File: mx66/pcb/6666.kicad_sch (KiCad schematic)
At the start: 145 parts, among them J1 Left side, J2 Right side, K1 100, K10 125, K11 100, K12 100, K13 100, K14 100, K15 125, K16 100, K17 100, K18 100, K19 100, K2 150, K20 125, K21 100, K22 100, K23 100, K24 100, K25 225, K26 100, K27 100, K28 100, K29 100, K3 175, K30 100, K31 100, K32 100, K33 100, K34 100, K35 100, K36 100, K37 100, K38 100, K39 100, K4 225, K40 100, K41 100, K42 100, K43 275, K44 100, K45 100, K46 100, K47 100, K48 125, K49 100, K5 125, K50 100, K51 100, K52 100, K53 125, K54 100, K55 100, K56 100, K57 100, K58 100, K59 100, K6 100, K60 100, K61 100, K62 200, K63 150, K64 225, K65 100, K66 100, K7 100, K8 100, K9 100, U1 MCU_ProMicro_13p, U2 MCU_ProMicro_13p

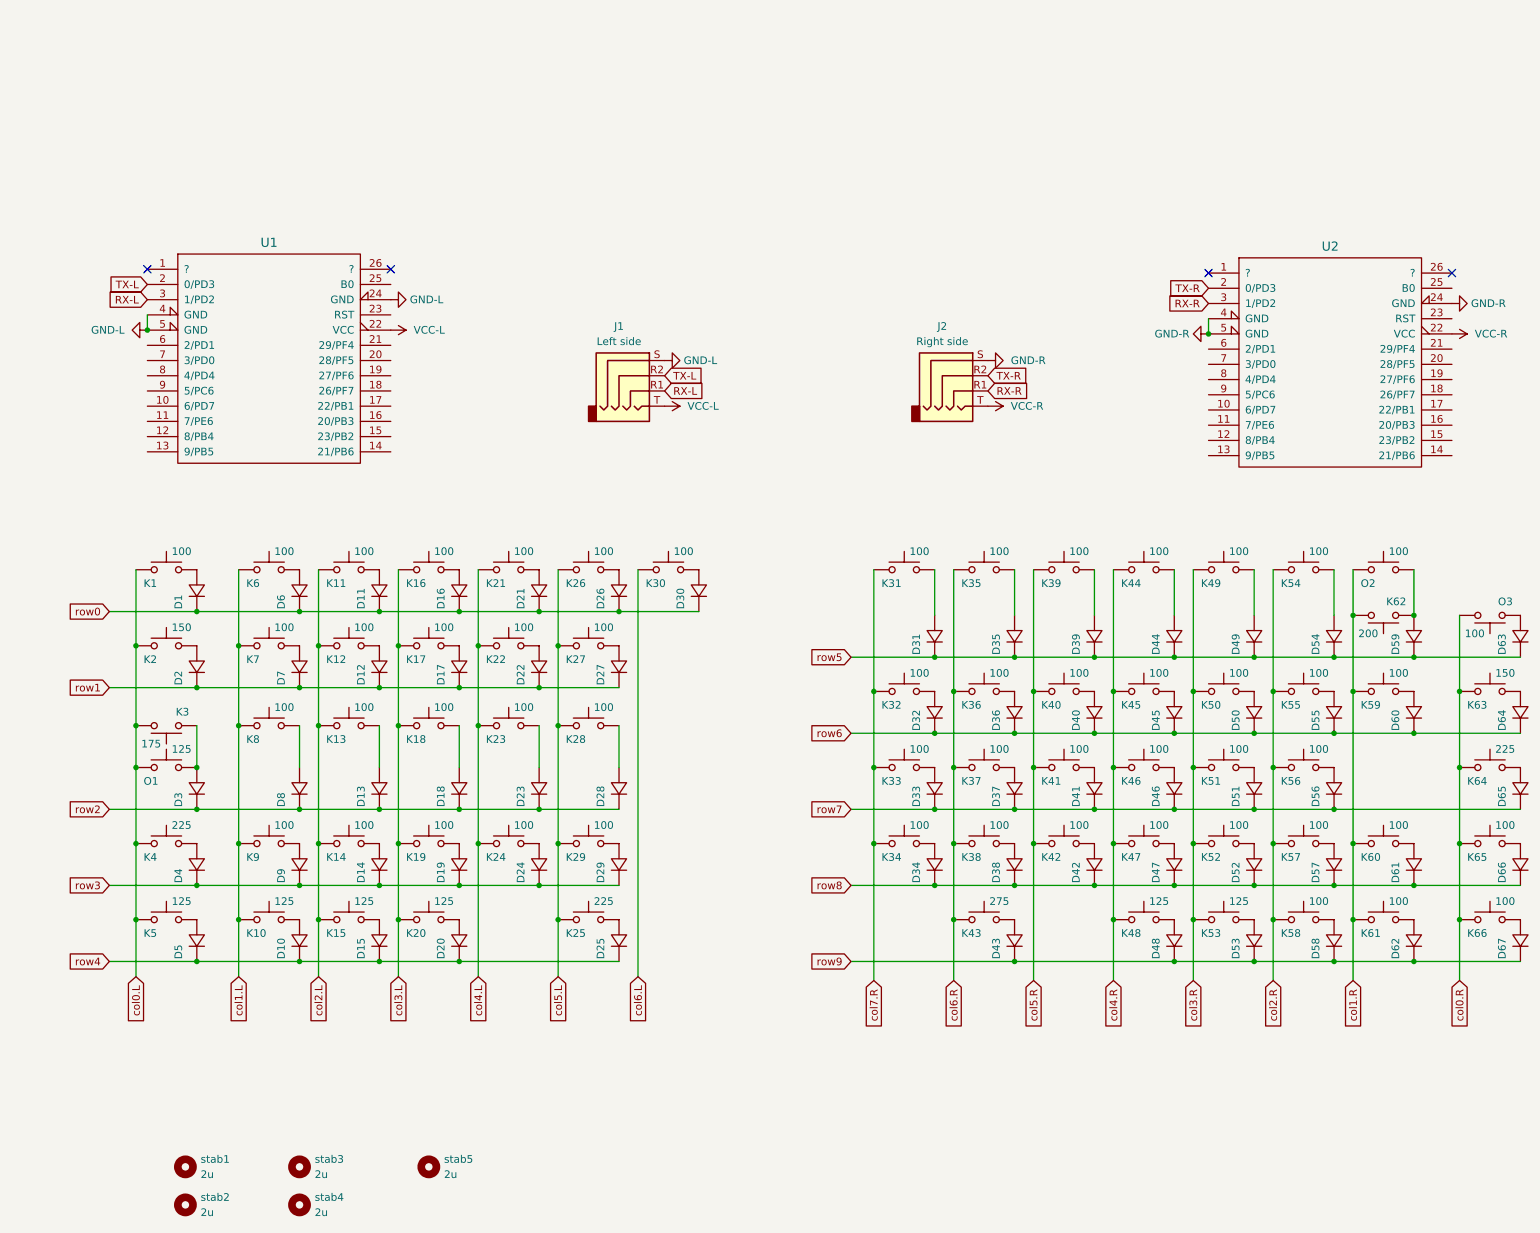
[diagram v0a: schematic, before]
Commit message: set pinout and layout
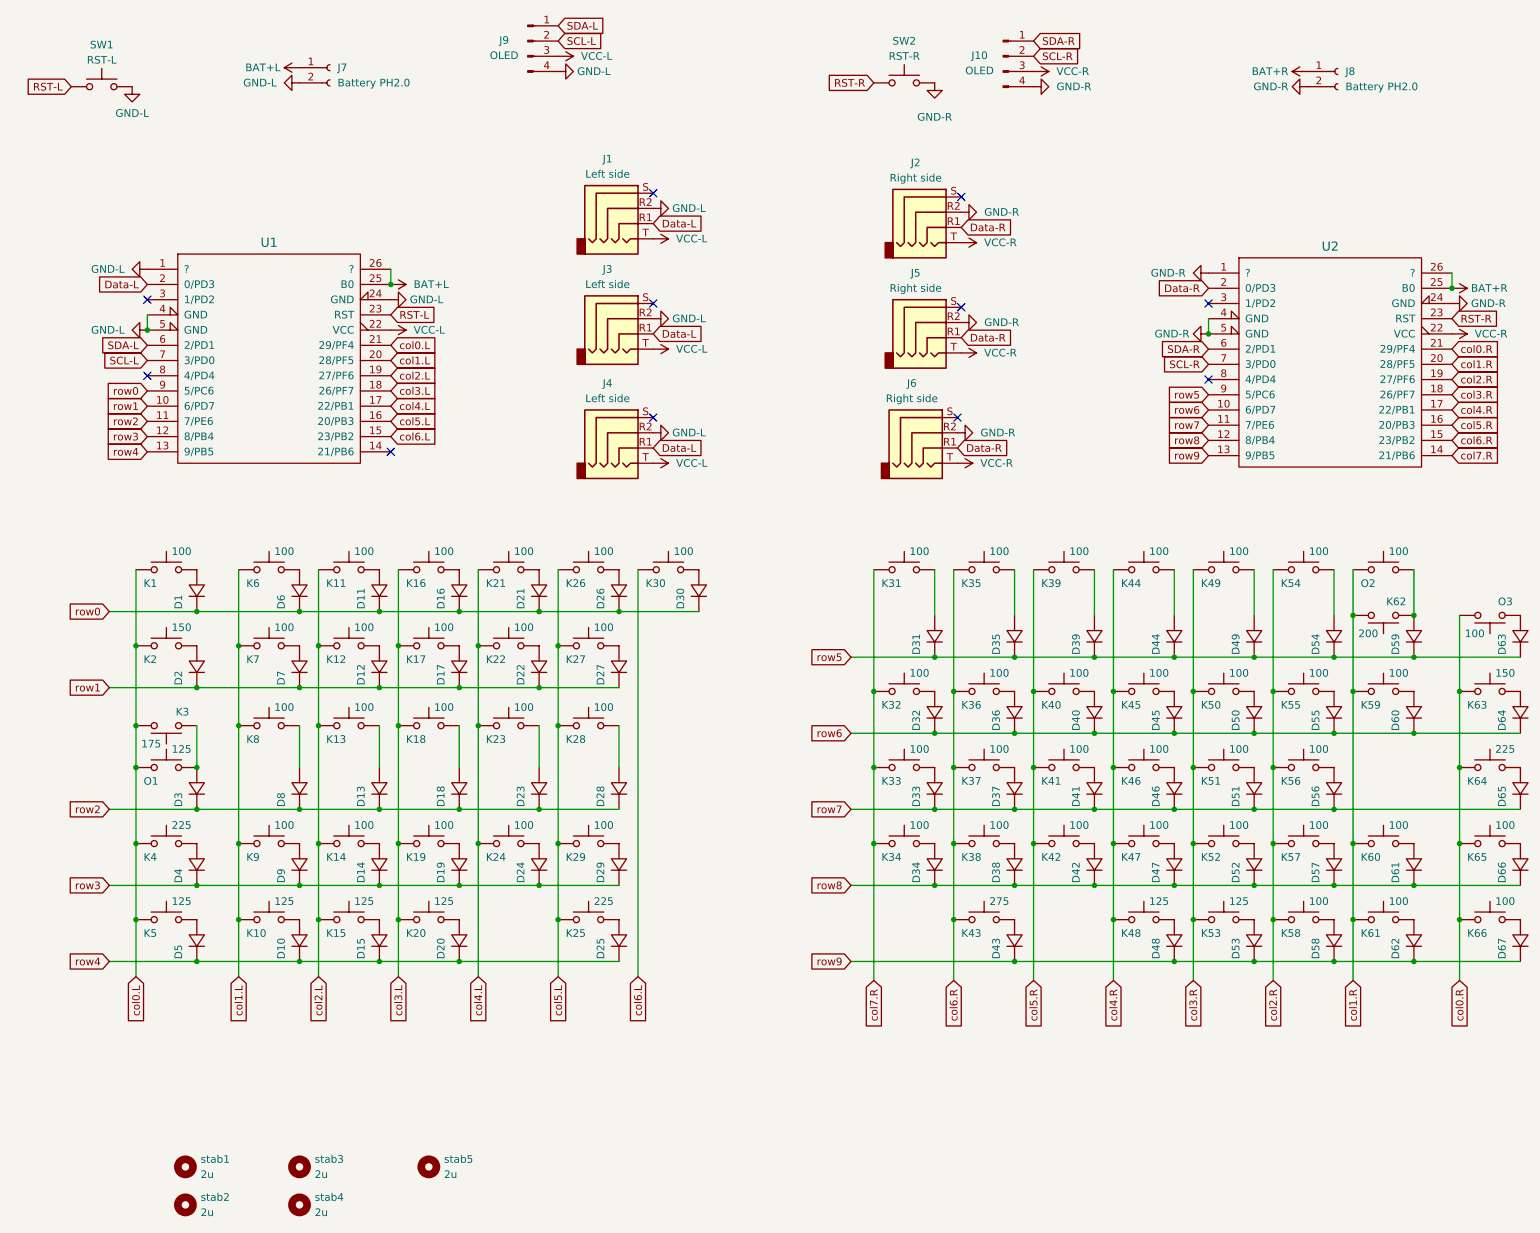
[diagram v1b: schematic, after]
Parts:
- added J10, J9: OLED, DreaM117er-keebLibrary:PinHeader_1x04_P2.54mm_Vertical, symbol Connector:Conn_01x04_Pin
- added J3, J4: Left side, DreaM117er-keebLibrary:TRRS-PJ-320A, symbol Connector_Audio:AudioJack4
- added J5, J6: Right side, DreaM117er-keebLibrary:TRRS-PJ-320A, symbol Connector_Audio:AudioJack4
- added J7, J8: Battery PH2.0, Connector_JST:JST_PH_S2B-PH-K_1x02_P2.00mm_Horizontal, symbol Connector:Conn_01x02_Socket
- added SW1: RST-L, DreaM117er-keebLibrary:ResetSW_1side, symbol Switch:SW_Push
- added SW2: RST-R, DreaM117er-keebLibrary:ResetSW_1side, symbol Switch:SW_Push
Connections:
- net GND-L: now also J1.R2, U1.1 (?), J3.R2, J4.R2, J7.2 (Pin_2), J9.4 (Pin_4), SW1.2; no longer J1.S
- net GND-R: now also J2.R2, U2.1 (?), J10.4 (Pin_4), J5.R2, J6.R2, J8.2 (Pin_2), SW2.2; no longer J2.S
- net VCC-L: now also J3.T, J4.T, J9.3 (Pin_3)
- net VCC-R: now also J10.3 (Pin_3), J5.T, J6.T
- net col0.L: now also U1.21 (29/PF4)
- net col0.R: now also U2.21 (29/PF4)
- net col1.L: now also U1.20 (28/PF5)
- net col1.R: now also U2.20 (28/PF5)
- net col2.L: now also U1.19 (27/PF6)
- net col2.R: now also U2.19 (27/PF6)
- net col3.L: now also U1.18 (26/PF7)
- net col3.R: now also U2.18 (26/PF7)
- net col4.L: now also U1.17 (22/PB1)
- net col4.R: now also U2.17 (22/PB1)
- net col5.L: now also U1.16 (20/PB3)
- net col5.R: now also U2.16 (20/PB3)
- net col6.L: now also U1.15 (23/PB2)
- net col6.R: now also U2.15 (23/PB2)
- net col7.R: now also U2.14 (21/PB6)
- net row0: now also U1.9 (5/PC6)
- net row1: now also U1.10 (6/PD7)
- net row2: now also U1.11 (7/PE6)
- net row3: now also U1.12 (8/PB4)
- net row4: now also U1.13 (9/PB5)
- net row5: now also U2.9 (5/PC6)
- net row6: now also U2.10 (6/PD7)
- net row7: now also U2.11 (7/PE6)
- net row8: now also U2.12 (8/PB4)
- net row9: now also U2.13 (9/PB5)
- net RST-R: now reaches U2.23 (RST)
- net RST-R: now also SW2.1
- net BAT+R: now reaches U2.25 (B0)
- net BAT+R: now also U2.26 (?), J8.1 (Pin_1)
- net SDA-R: now reaches U2.6 (2/PD1)
- net SDA-R: now also J10.1 (Pin_1)
- net SCL-R: now reaches U2.7 (3/PD0)
- net SCL-R: now also J10.2 (Pin_2)
- net RST-L: now reaches U1.23 (RST)
- net RST-L: now also SW1.1
- net BAT+L: now reaches U1.25 (B0)
- net BAT+L: now also U1.26 (?), J7.1 (Pin_1)
- net SDA-L: now reaches U1.6 (2/PD1)
- net SDA-L: now also J9.1 (Pin_1)
- net SCL-L: now reaches U1.7 (3/PD0)
- net SCL-L: now also J9.2 (Pin_2)
- net RX-L: no longer names the net of U1.3 (1/PD2)
- net RX-L: no longer J1.R1
- net RX-R: no longer names the net of U2.3 (1/PD2)
- net RX-R: no longer J2.R1
- net TX-L renamed Data-L
- net Data-L: now also J1.R1, J3.R1, J4.R1; no longer J1.R2
- net TX-R renamed Data-R
- net Data-R: now also J2.R1, J5.R1, J6.R1; no longer J2.R2
- no-connect marks 4 -> 11
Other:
- moved on the sheet: J1, J2
